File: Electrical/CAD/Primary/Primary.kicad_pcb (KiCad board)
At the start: 2 copper layers, 0 parts

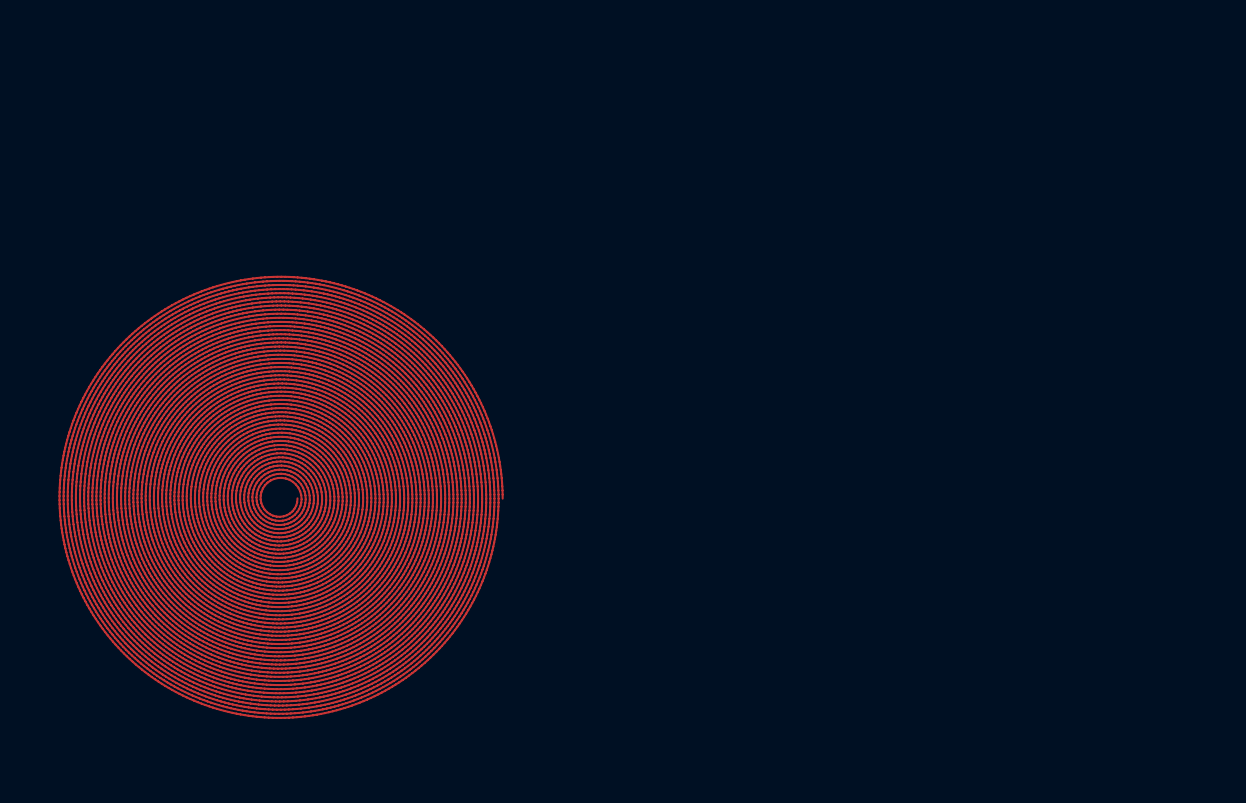
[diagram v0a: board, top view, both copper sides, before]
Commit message: Mid episode 10 commit.
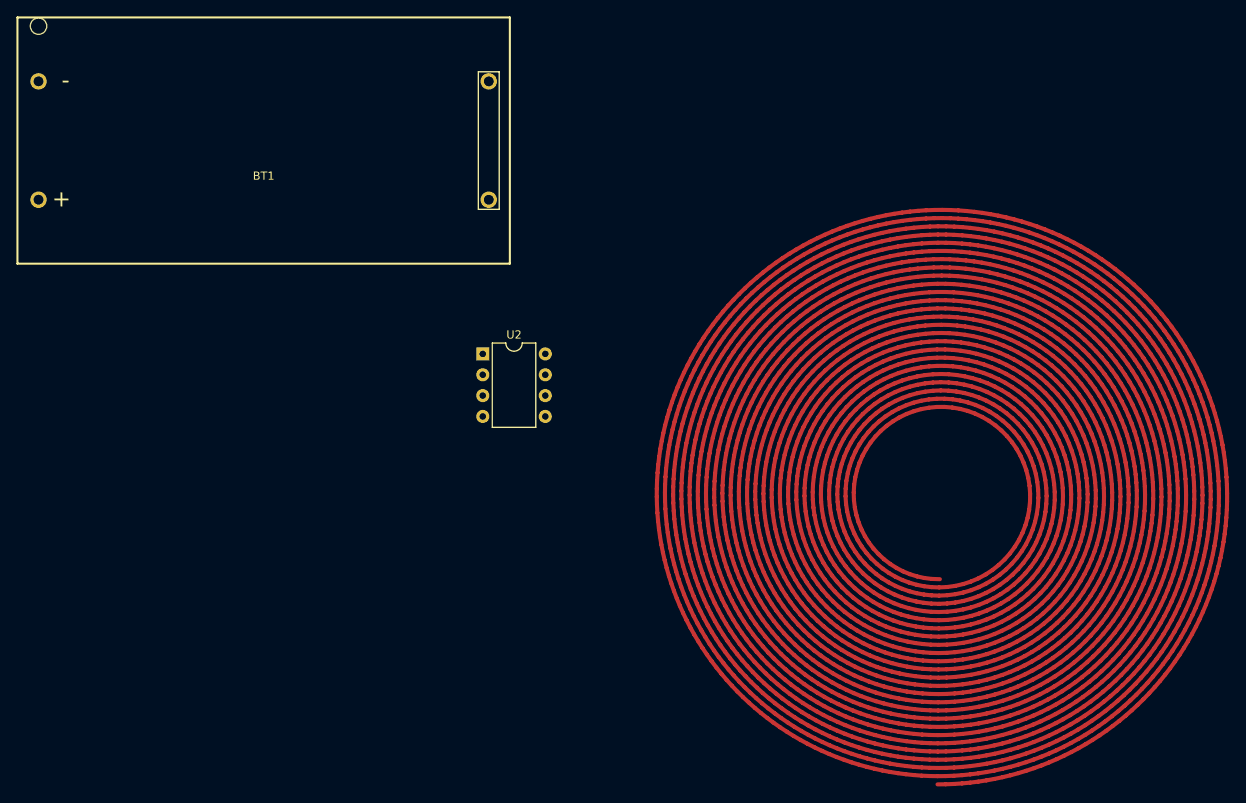
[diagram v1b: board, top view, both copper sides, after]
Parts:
- added BT1: 2x_Battery_Cell, WirelessPower:Keystone_Dual_AA_Holder, F.Cu at (98.0, 56.4)
- added U2: MCP6282, Package_DIP:DIP-8_W7.62mm, F.Cu at (124.7, 82.4)
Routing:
- net (no net): track 4594.4 -> 3573.6 mm
